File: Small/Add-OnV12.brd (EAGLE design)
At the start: 18.1 x 17.6 mm, 6 parts, among them X1 1501_03

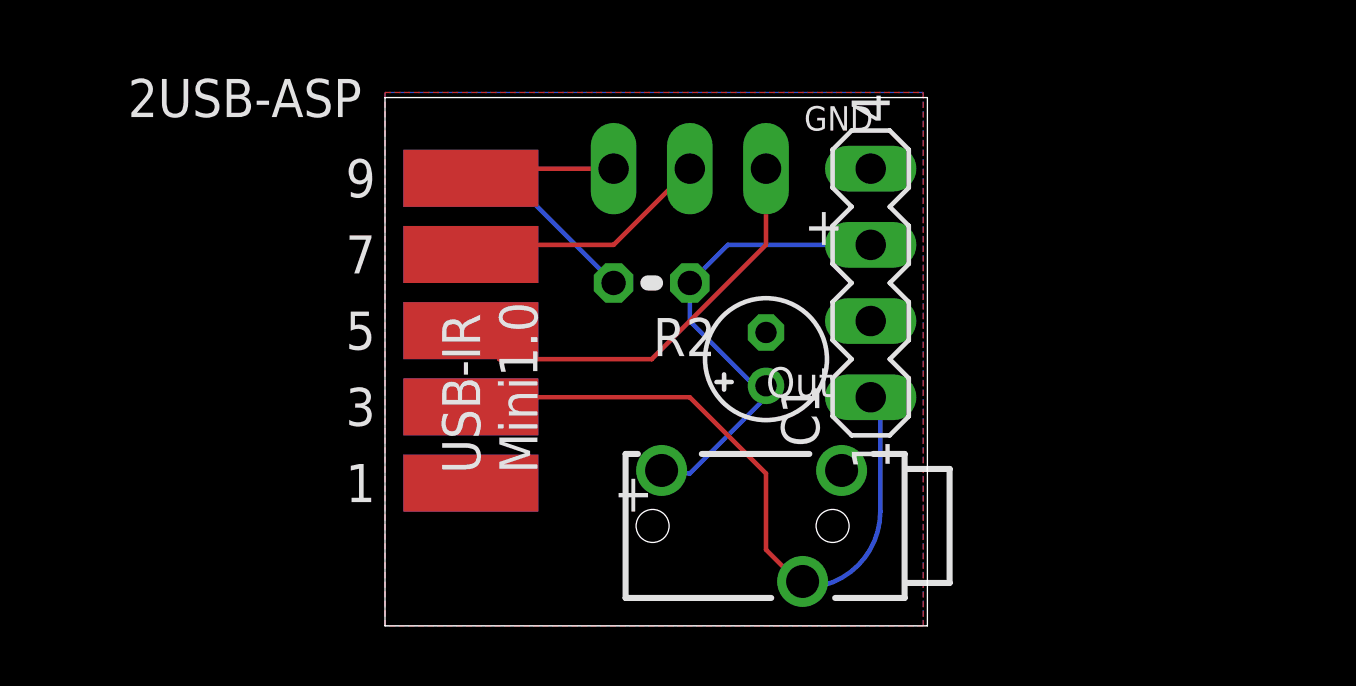
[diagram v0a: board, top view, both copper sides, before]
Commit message: Final Layout
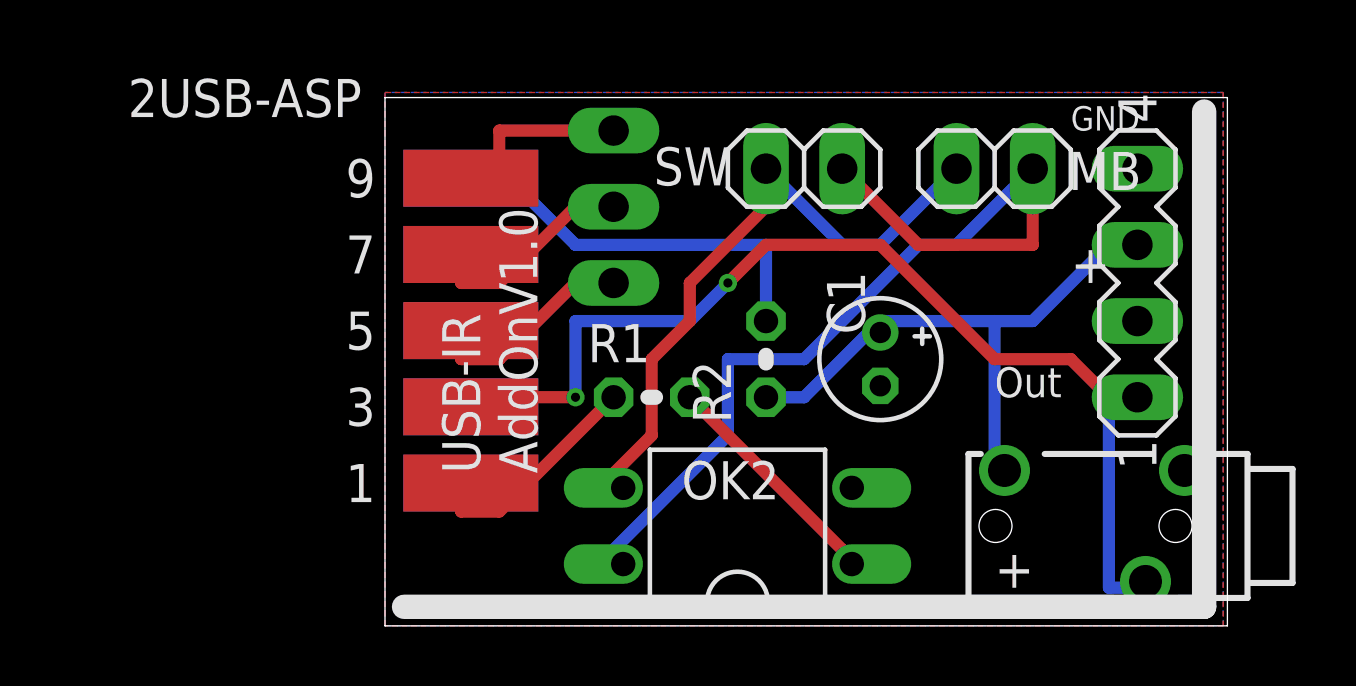
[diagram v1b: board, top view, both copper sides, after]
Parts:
- added MB, SW: (no value), pinhead:1X02
- added OK2: PC817, optocoupler:DIL04
- added R1: 100, rcl:0204V
- moved X1 11.4 mm to (26.4, 3.33)
- moved SV1 8.89 mm to (25.1, 11.4)
- moved R2 4.58 mm to (12.7, 8.89), turned to 90 degrees
- moved C1 3.81 mm to (16.5, 8.89), turned to 270 degrees
- moved FREI 2.84 mm to (7.62, 14.0), turned to 270 degrees
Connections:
- new net N$2: OK2.1, R1.2
- new net N$3: MB.2, OK2.4, SW.1
- new net N$4: MB.1, OK2.3, SW.2
- net GND: now also OK2.2
- net MISO: now also R1.1
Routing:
- net N$3: track 0.00 -> 31.2 mm
- net N$4: track 0.00 -> 21.3 mm
- net SCK: track 23.4 -> 36.8 mm, vias 0 -> 2
- net MISO: track 0.00 -> 8.38 mm
- net N$2: track 0.00 -> 7.76 mm
- net RST: track 15.3 -> 7.85 mm
- net VCC: track 6.39 -> 13.5 mm
- net N$1: track 17.0 -> 20.7 mm
- net MOSI: track 4.81 -> 6.08 mm
- net NC: track 8.40 -> 7.85 mm
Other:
- board size 18.1 x 17.6 mm -> 28.1 x 17.6 mm
- board text added: "USB-IR AddOnV1.0"
- board text removed: "USB-IR Mini1.0"
